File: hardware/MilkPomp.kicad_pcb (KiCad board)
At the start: 2 copper layers, 137 x 65 mm, 76 parts, among them J1 Screw_Terminal_01x06, J2 BOOT, J3 Conn_01x04_Male, J4 Conn_Board, J5 Conn_Display, J6 PWR INPUT, K1 G5LE-1, Q1 BC847, SW1 SW_IO, SW2 SW_START, SW3 SW_MODE, U1 STM32F103C8Tx, U2 TLP291, U3 HDSP-7403, U4 TPS7A4901DGNT, U5 LD1085D2M-R, Y1 8MHz, Y2 32KHz

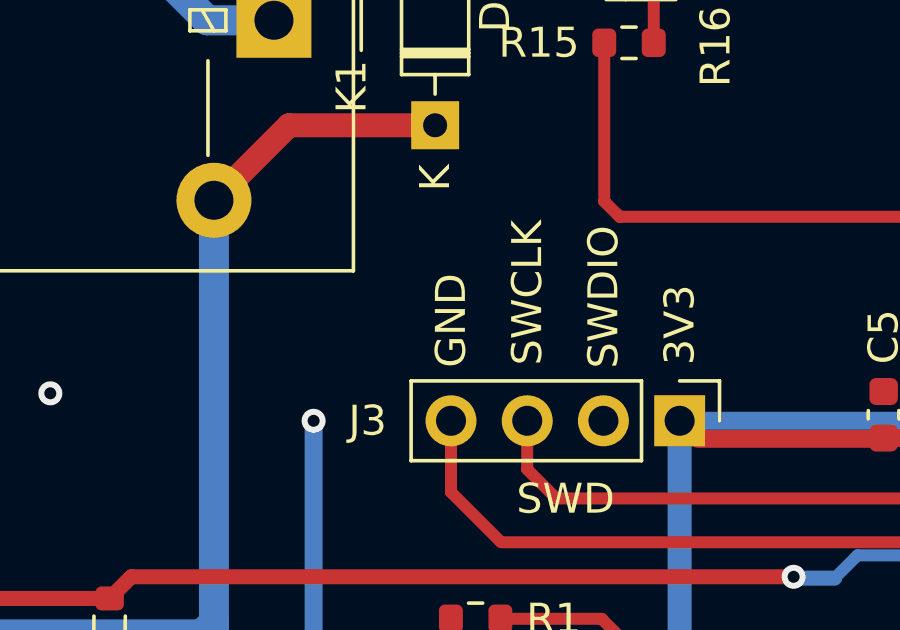
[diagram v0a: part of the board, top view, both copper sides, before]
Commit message: yeni seyler eklendi
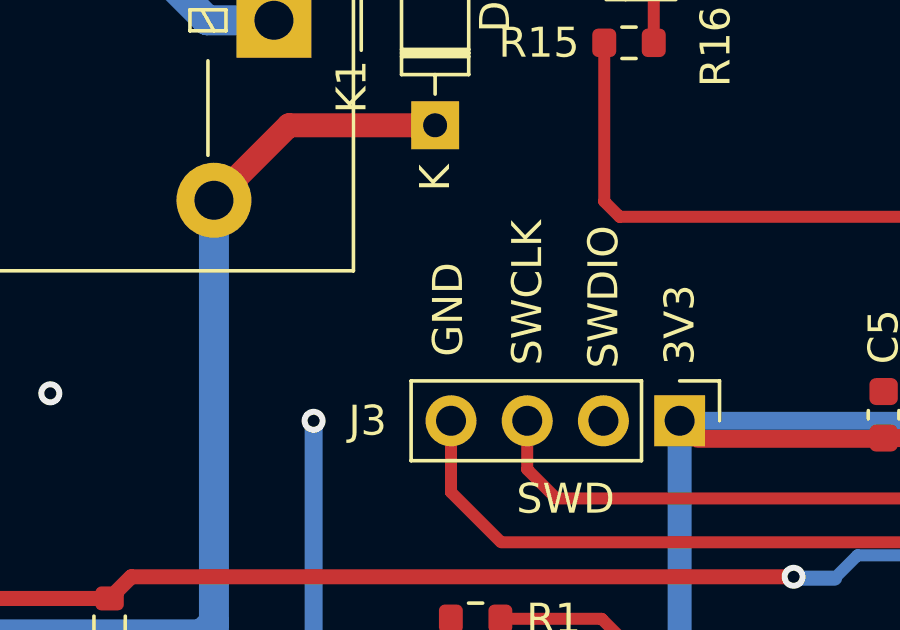
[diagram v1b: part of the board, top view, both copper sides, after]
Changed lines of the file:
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@@
     (effects (font (size 1 1) (thickness 0.15)))
   )
-  (gr_text "GND" (at 129.7904 100.341543 90) (layer "F.SilkS")
+  (gr_text "GND" (at 129.6924 99.9744 90) (layer "F.SilkS")
     (effects (font (size 1 1) (thickness 0.15)))
   )
